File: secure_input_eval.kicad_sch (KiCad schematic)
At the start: 64 parts, among them CON1_STLINK1 ST-LINK, J10 masa pomiarowa, J18_CPU_CON1 Conn_CPU, J19 masa pomiarowa, J23 masa pomiarowa, J24 masa pomiarowa, J25 masa pomiarowa, J26 masa pomiarowa, J27_USART3 USART, J28_PIN14_PA7 TOUCH_SINGLE, J29_D+_PIN23_PA12 D+_PP, J2_SD_SPI1 MEM2085-00-115-00-A_REV0.2, J30_D-_PIN22_PA11 D-_PP, J31_CS_PP_PIN7_PA0 CS_PP_PIN7_PA0, J32_MOSI_PIN9_PA2 MOSI_PP, J33_MISO_PP_PIN13_PA6 MISO_PP_PIN13_PA6, J34_SCK_PP_PIN8_PA1 SCK_PP_PIN8_PA1, J35_SCL_PP_PIN19_PA9 SCL_PP_PIN19_PA9, J36_SDA_PP_PIN1_PB9 SDA_PP_PIN1_PB9, J3_SWO_NC1 SWO NC, J7 masa pomiarowa, J9 masa pomiarowa, SW1_PIN11_PA4 B3U-3000P, SW2_PIN32_PB8 B3U-3000P, SW3_PIN31_PB7 B3U-3000P, SW4_PIN26_PA15 B3U-3000P, SW5_TCH__PIN12_PA5 sensor dotykowy_PIN12_PA5, SW6_PIN25_PA14 BOOT0, U1 STM32G0B1KETx, U2 LD1117-3.3

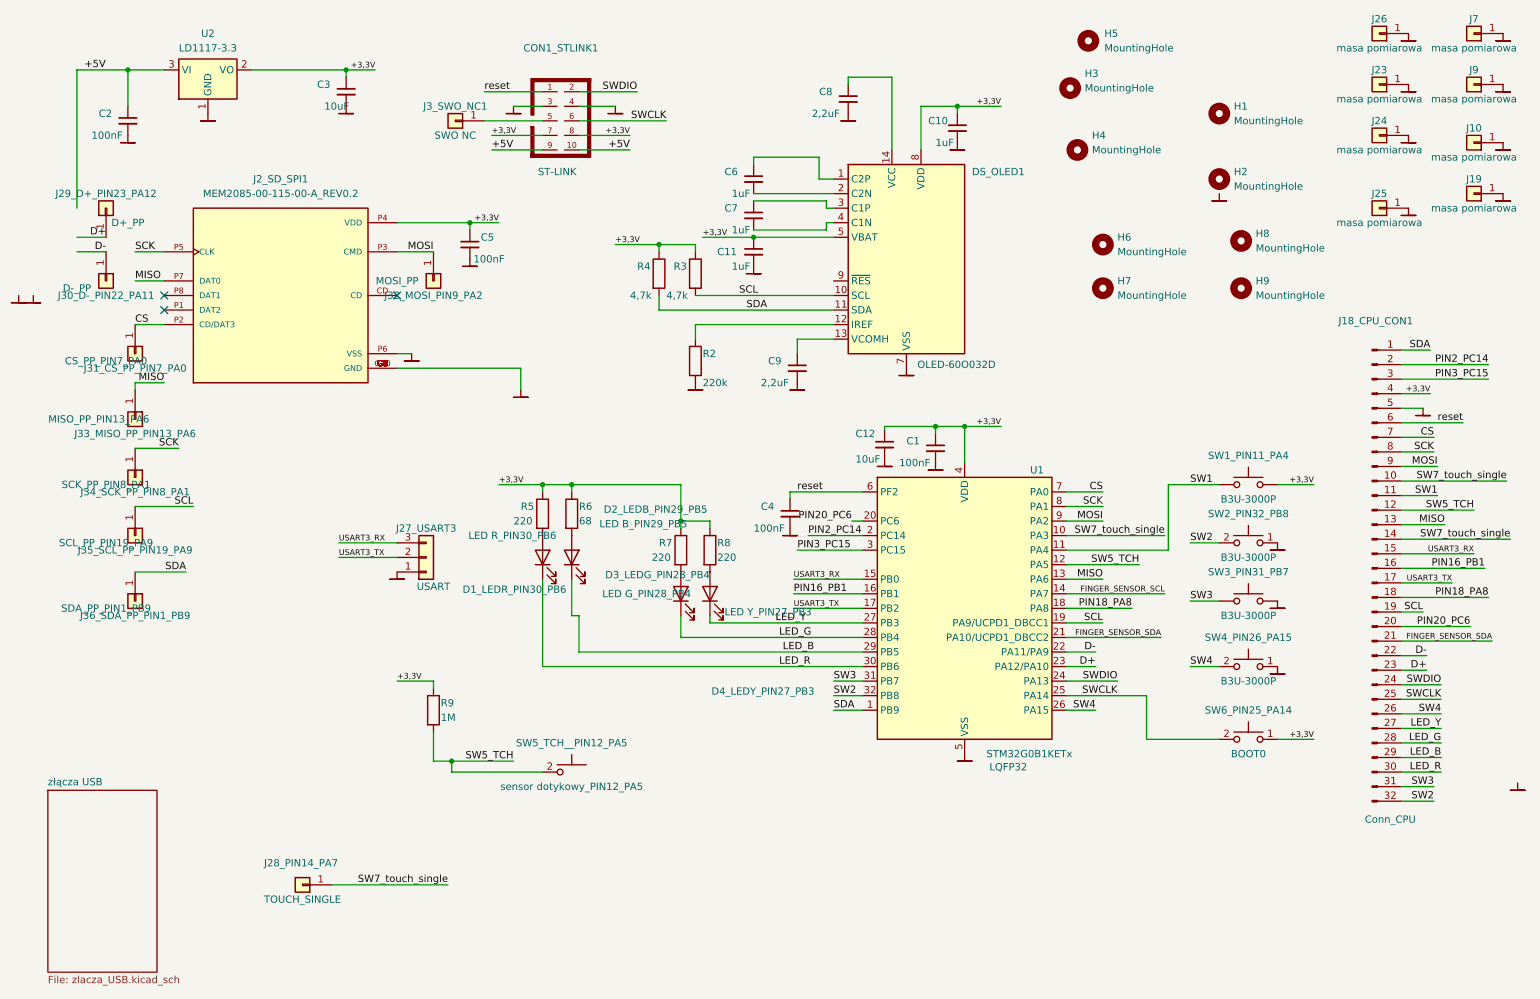
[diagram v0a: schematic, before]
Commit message: TITLES&SUBTITLES POSITIONS & NAMES.
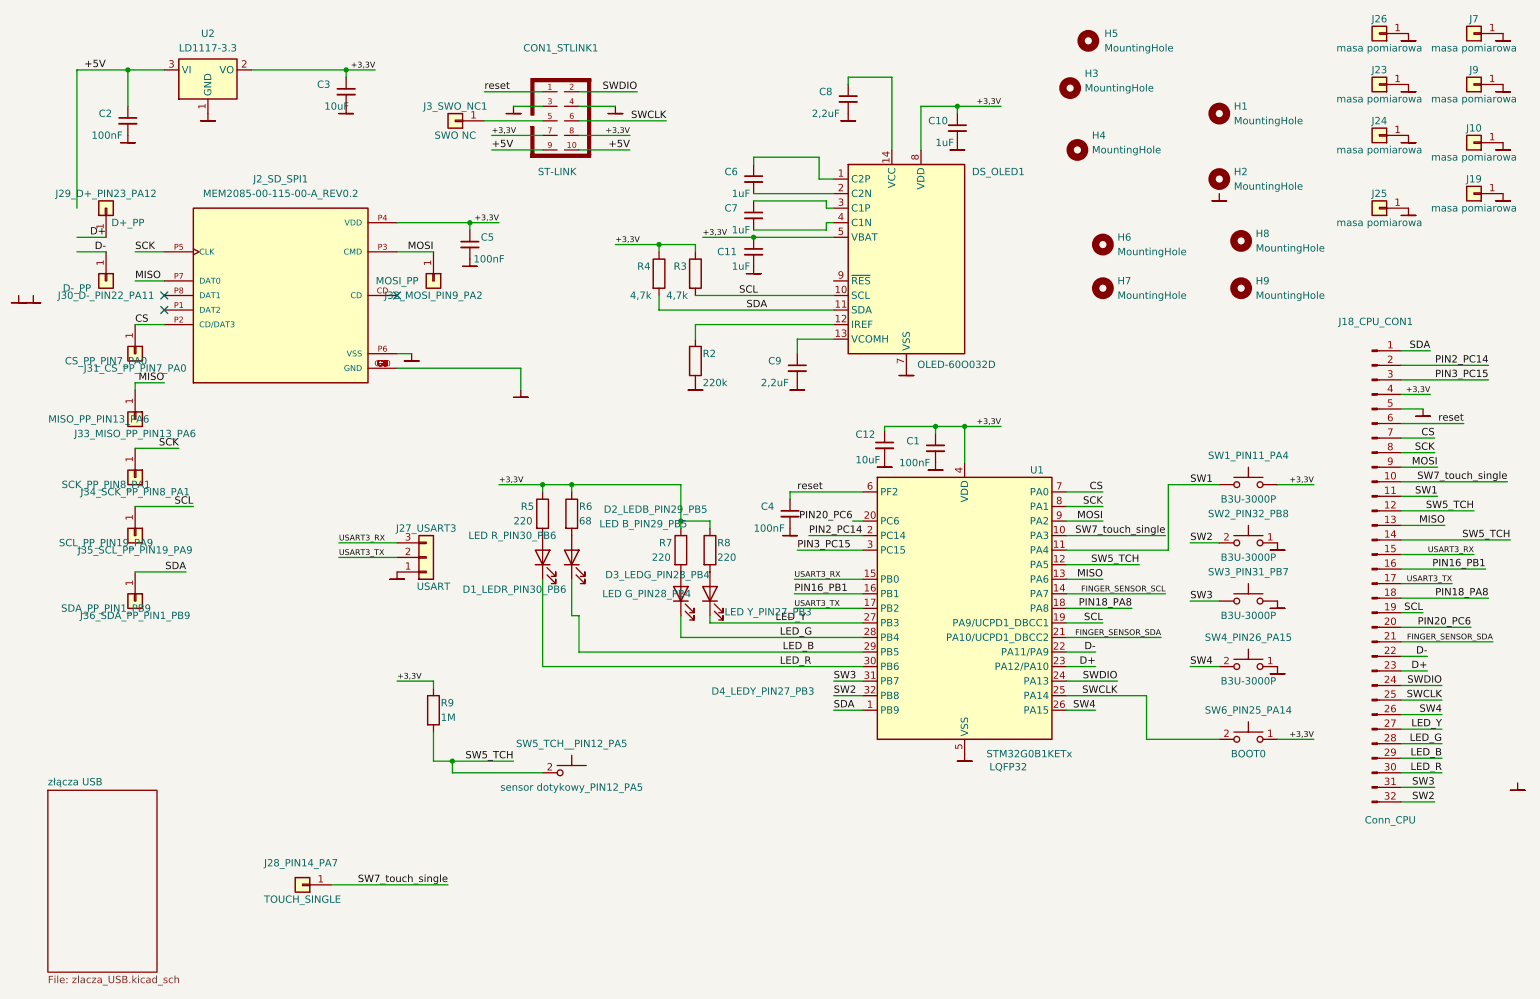
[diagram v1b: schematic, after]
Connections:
- net SW5_TCH: now also J18_CPU_CON1.14 (Pin_14)
- net SW7_touch_single: no longer J18_CPU_CON1.14 (Pin_14)
